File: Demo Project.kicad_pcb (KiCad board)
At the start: 4 copper layers, 60 x 75 mm, 133 parts, among them J1 PWR, J2 SMA_Conn, J4 Term, J5 RS485, J6 RS422, J7 Term, J8 ICSP_Prog_Header, Q1 BSS84, Q2 BSS84, SW1 RST, SW2 Mode, SW3 RST, U1 LMR54406DBVR, U2 B0505S-1WR3, U3 TLV75733PDBV, U4 CORE1262-868M, U5 THVD1452DGSR, U6 THVD1452DGSR, U7 ISO6762DWR, U8 PIC18F67K22-I/PT, Y1 20MHz

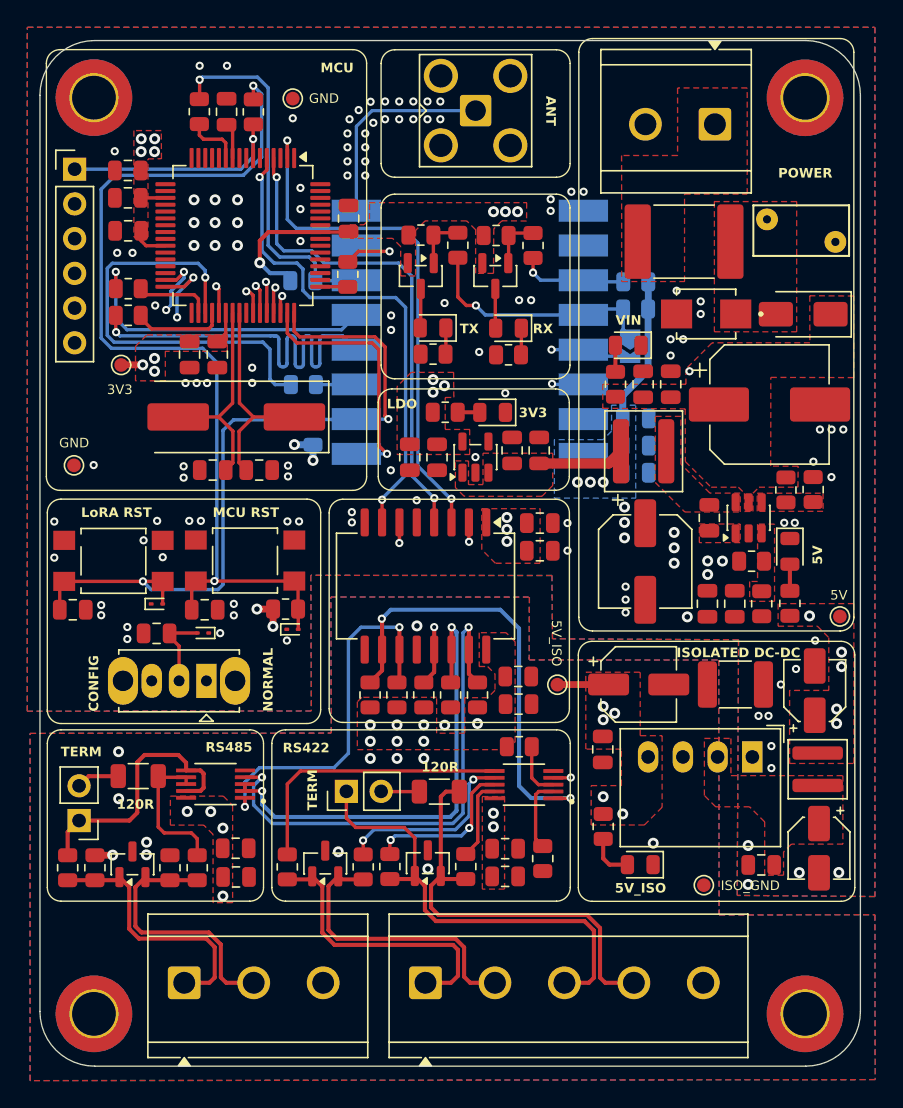
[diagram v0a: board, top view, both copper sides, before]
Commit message: reverted back to og files
[local revision r5 4274e03a1d0e]
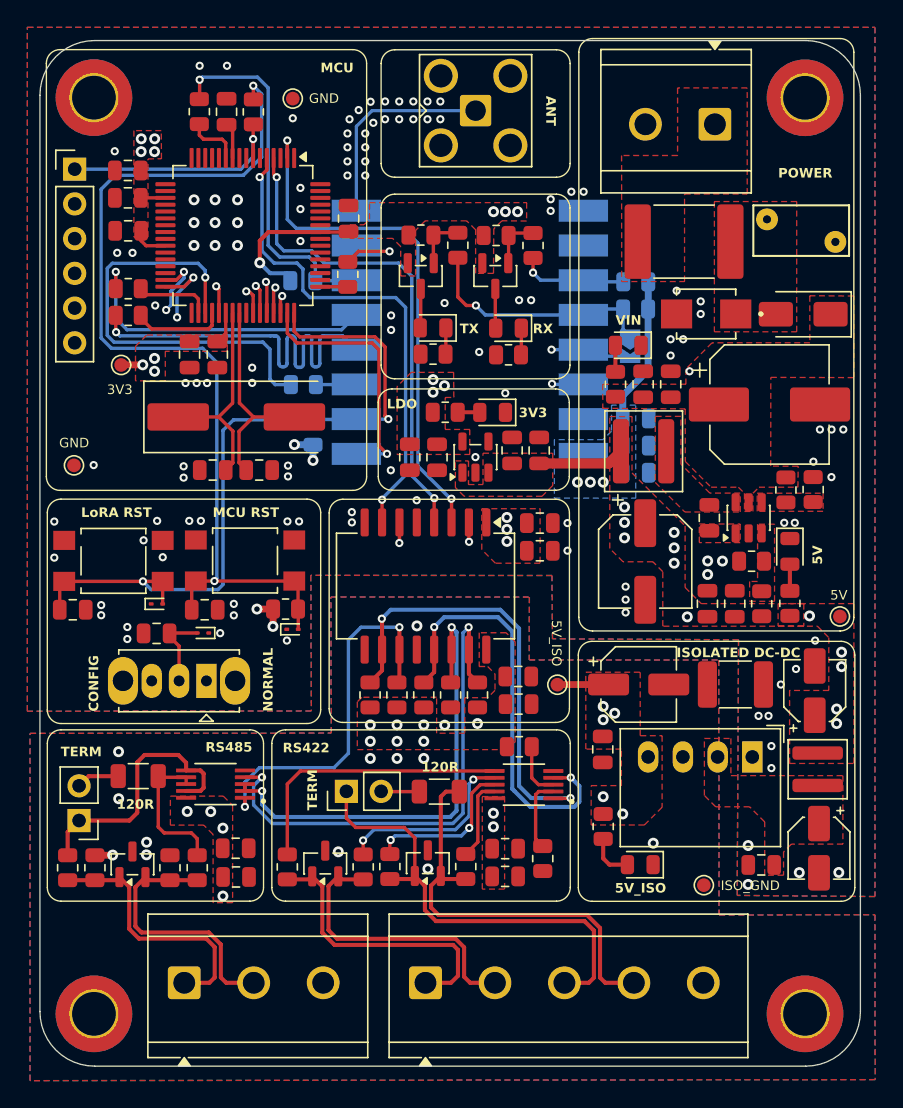
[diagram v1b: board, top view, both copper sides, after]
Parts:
- turned Y1 to 0 degrees
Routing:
- net RS422_Tx: track 5.65 -> 31.3 mm

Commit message: testing plugin
[local revision r3 cb60daacd4a3]
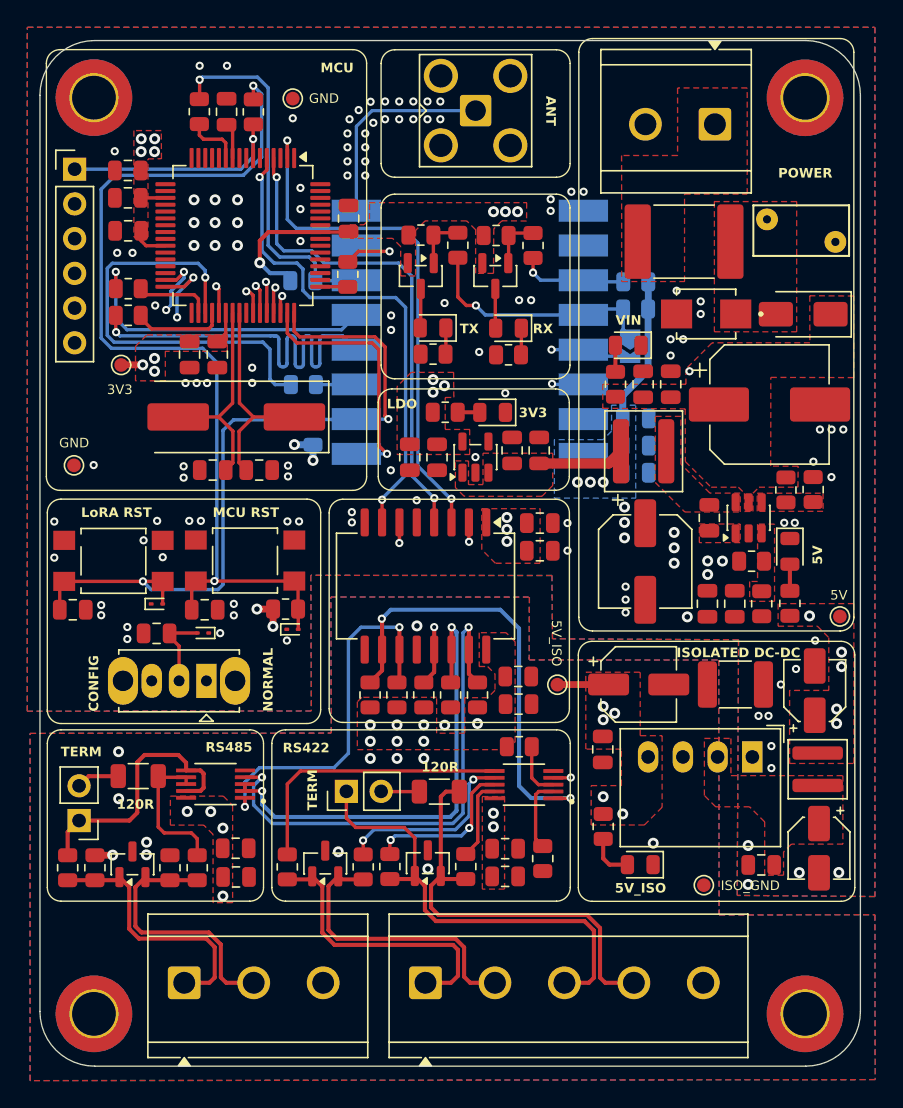
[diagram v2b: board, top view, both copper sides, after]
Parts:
- turned Y1 to 180 degrees
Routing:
- net RS422_Tx: track 31.3 -> 5.65 mm
